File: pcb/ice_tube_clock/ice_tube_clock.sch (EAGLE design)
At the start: 11 parts, among them IC1 7805TV

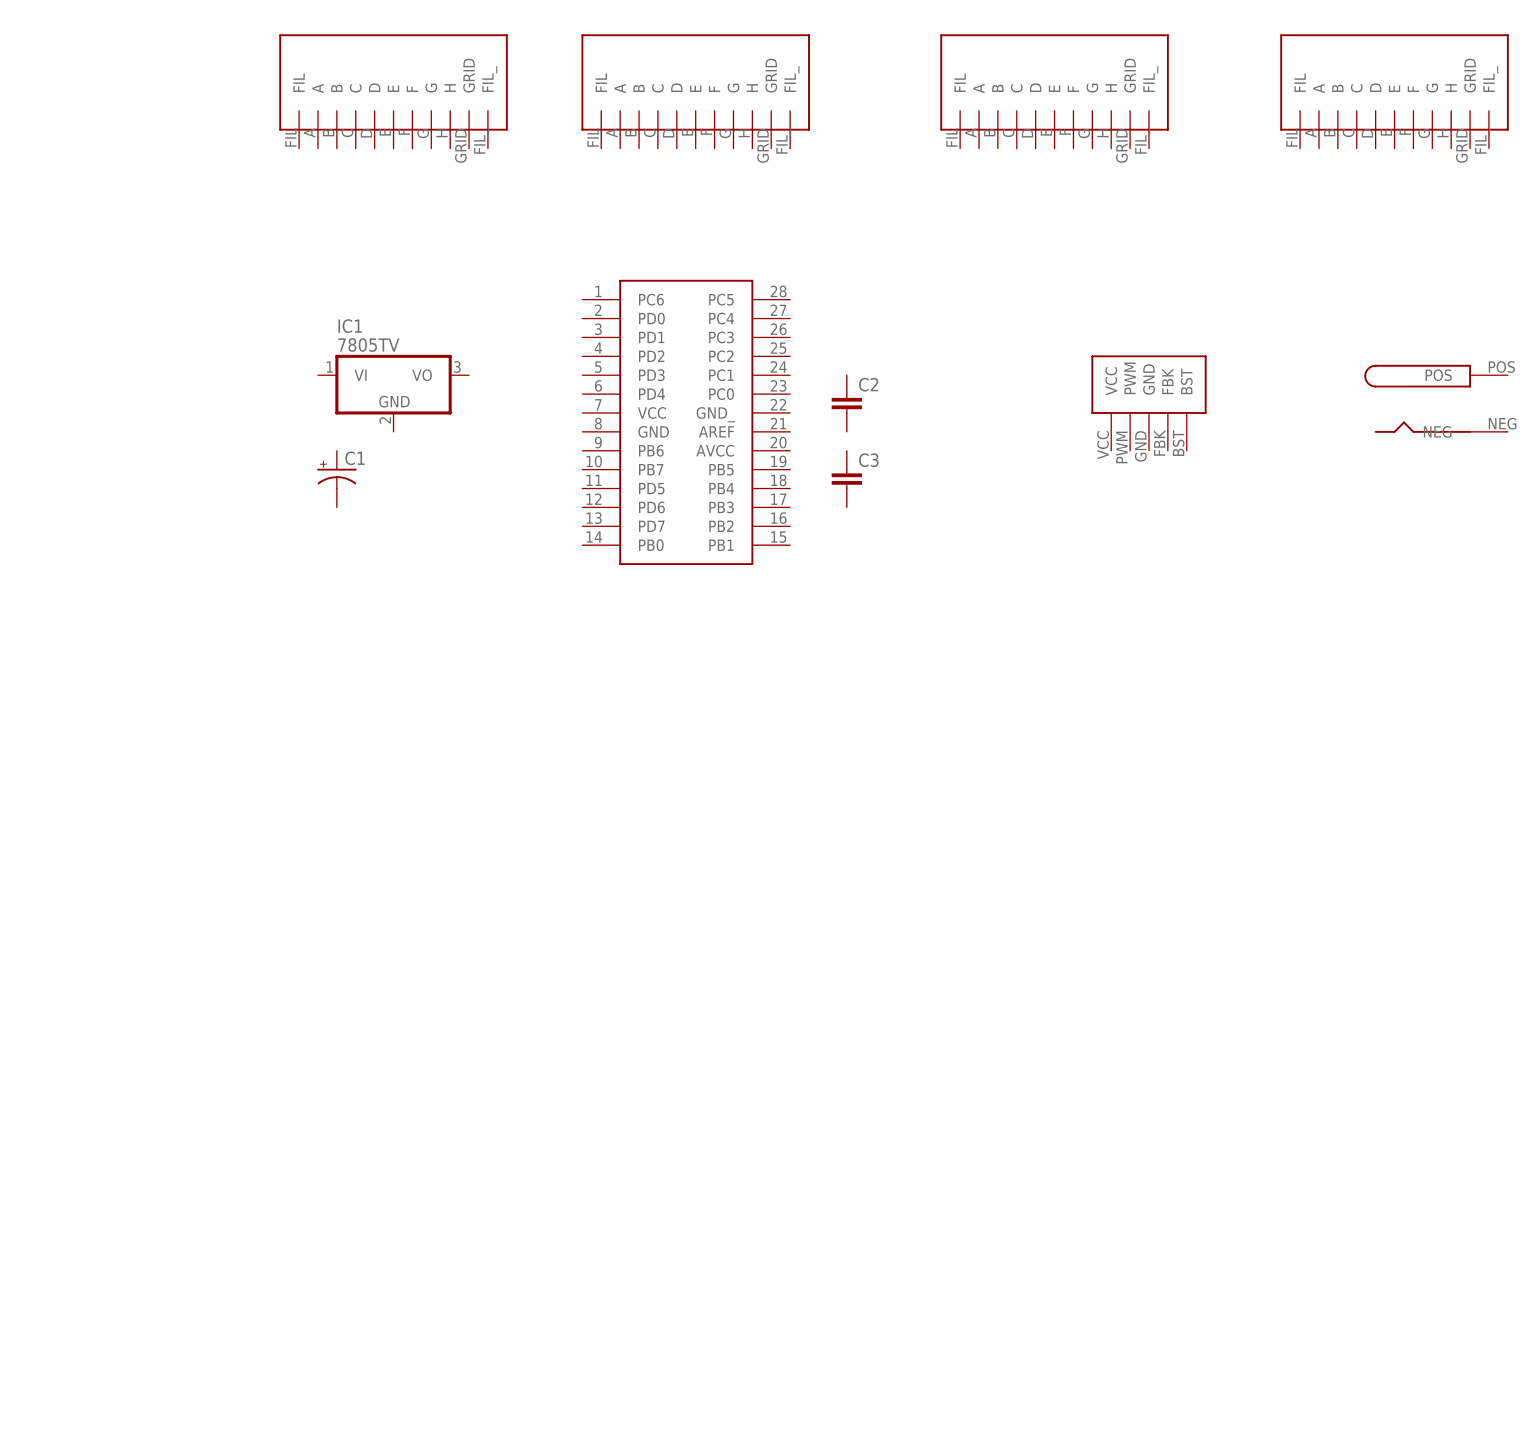
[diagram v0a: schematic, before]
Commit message: I thought I committed all this stuff
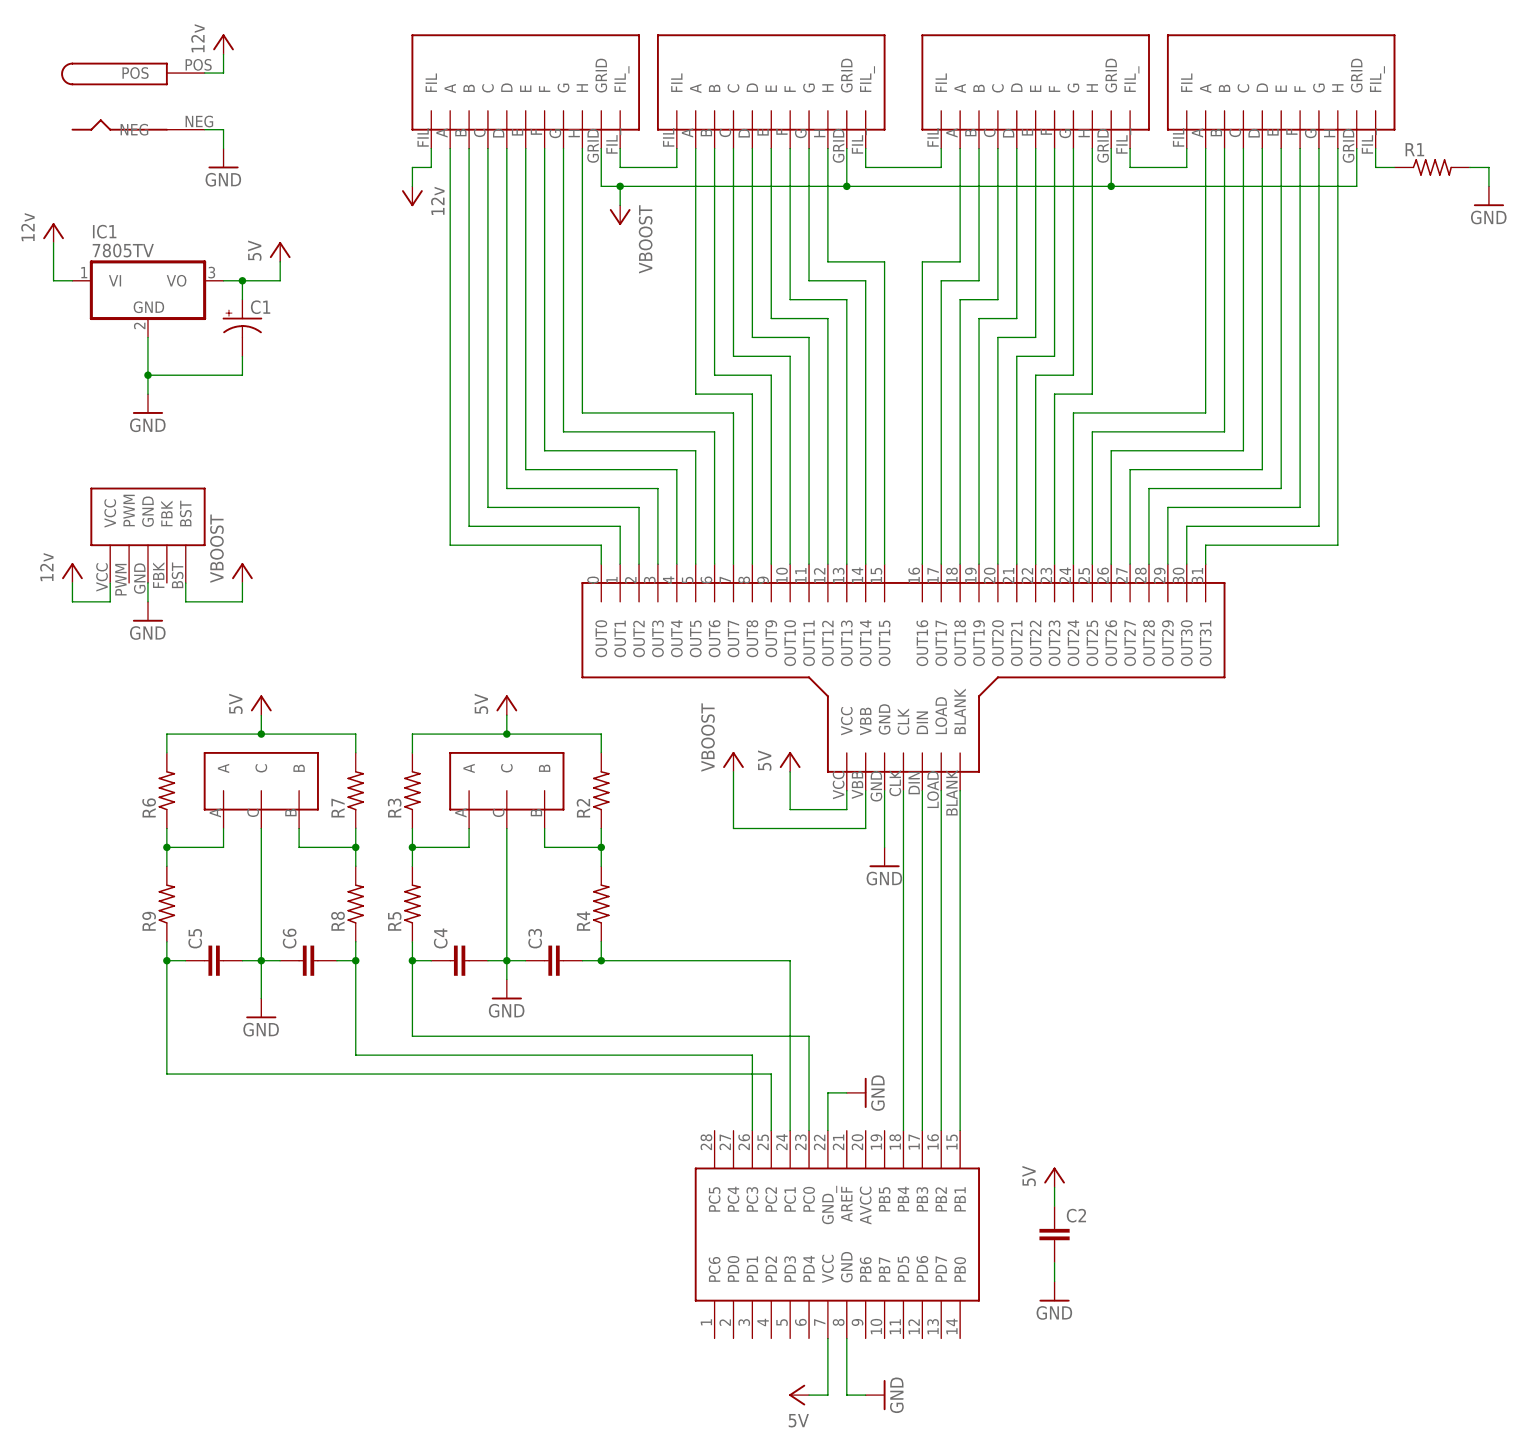
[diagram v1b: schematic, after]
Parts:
- added C4, C5, C6: (no value), SparkFun-Capacitors:0.1UF-50V-20%(PTH)KIT-EZ
- added R1, R2, R3, R4, R5, R6, R7, R8, R9: (no value), resistor:R-US_0204/7
- added U$10, U$9: PEL12S, boztalay:PEL12S
- added U$8: VFD-DRIVER-CARRIER, boztalay:VFD-DRIVER-CARRIER
- U$1: value ATMEGA168-ZIF-28 -> ATMEGA168-DIP28; device boztalay:ATMEGA168-ZIF-28 -> boztalay:ATMEGA168-DIP28
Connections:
- new net +12V: IC1.VI, U$2.VCC, U$3.FIL, U$7.POS
- new net +5V: C1.+, C2.1, IC1.VO, R2.2, R3.2, R6.2, R7.2, U$1.VCC, U$8.VCC
- new net ET: C4.1, R5.1, U$1.PC0
- new net GND: C1.-, C2.2, C3.1, C4.2, C5.2, C6.1, IC1.GND, R1.2, U$1.GND, U$1.GND_, U$10.C, U$2.GND, U$7.NEG, U$8.GND, U$9.C
- new net N$1: U$3.FIL_, U$4.FIL
- new net N$10: U$3.G, U$8.OUT6
- new net N$11: U$3.H, U$8.OUT7
- new net N$13: U$4.A, U$8.OUT8
- new net N$14: U$4.B, U$8.OUT9
- new net N$15: U$4.C, U$8.OUT10
- new net N$16: U$4.D, U$8.OUT11
- new net N$17: U$4.E, U$8.OUT12
- new net N$18: U$4.F, U$8.OUT13
- new net N$19: U$4.G, U$8.OUT14
- new net N$2: U$4.FIL_, U$5.FIL
- new net N$20: U$4.H, U$8.OUT15
- new net N$21: U$6.H, U$8.OUT31
- new net N$22: U$6.G, U$8.OUT30
- new net N$23: U$6.F, U$8.OUT29
- new net N$24: U$6.E, U$8.OUT28
- new net N$25: U$6.D, U$8.OUT27
- new net N$26: U$6.C, U$8.OUT26
- new net N$27: U$6.B, U$8.OUT25
- new net N$28: U$6.A, U$8.OUT24
- new net N$29: U$5.H, U$8.OUT23
- new net N$3: U$5.FIL_, U$6.FIL
- new net N$30: U$5.G, U$8.OUT22
- new net N$31: U$5.F, U$8.OUT21
- new net N$32: U$5.E, U$8.OUT20
- new net N$33: U$5.D, U$8.OUT19
- new net N$34: U$5.C, U$8.OUT18
- new net N$35: U$5.B, U$8.OUT17
- new net N$36: U$5.A, U$8.OUT16
- new net N$37: R1.1, U$6.FIL_
- new net N$38: U$1.PB1, U$8.BLANK
- new net N$39: U$1.PB2, U$8.LOAD
- new net N$4: U$3.A, U$8.OUT0
- new net N$40: U$1.PB3, U$8.DIN
- new net N$41: U$1.PB4, U$8.CLK
- new net N$43: C3.2, R4.1, U$1.PC1
- new net N$44: R3.1, R5.2, U$10.A
- new net N$45: R6.1, R9.2, U$9.A
- new net N$46: R7.1, R8.2, U$9.B
- new net N$47: R2.1, R4.2, U$10.B
- new net N$48: C5.1, R9.1, U$1.PC2
- new net N$49: C6.2, R8.1, U$1.PC3
- new net N$5: U$3.B, U$8.OUT1
- new net N$6: U$3.C, U$8.OUT2
- new net N$7: U$3.D, U$8.OUT3
- new net N$8: U$3.E, U$8.OUT4
- new net N$9: U$3.F, U$8.OUT5
- new net VBOOST: U$2.BST, U$3.GRID, U$4.GRID, U$5.GRID, U$6.GRID, U$8.VBB
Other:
- moved on the sheet: C1, C2, C3, IC1
